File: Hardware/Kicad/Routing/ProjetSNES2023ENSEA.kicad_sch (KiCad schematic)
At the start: 43 parts, among them J1 Conn_01x07_Socket, Q1 2N7002, Q2 2N7002, Q3 2N7002, SW1 SW_Push, U1 NRF24L01, U2 AMS1117-3.3, U3 STM32L412KBTx, Y1 16 MHz

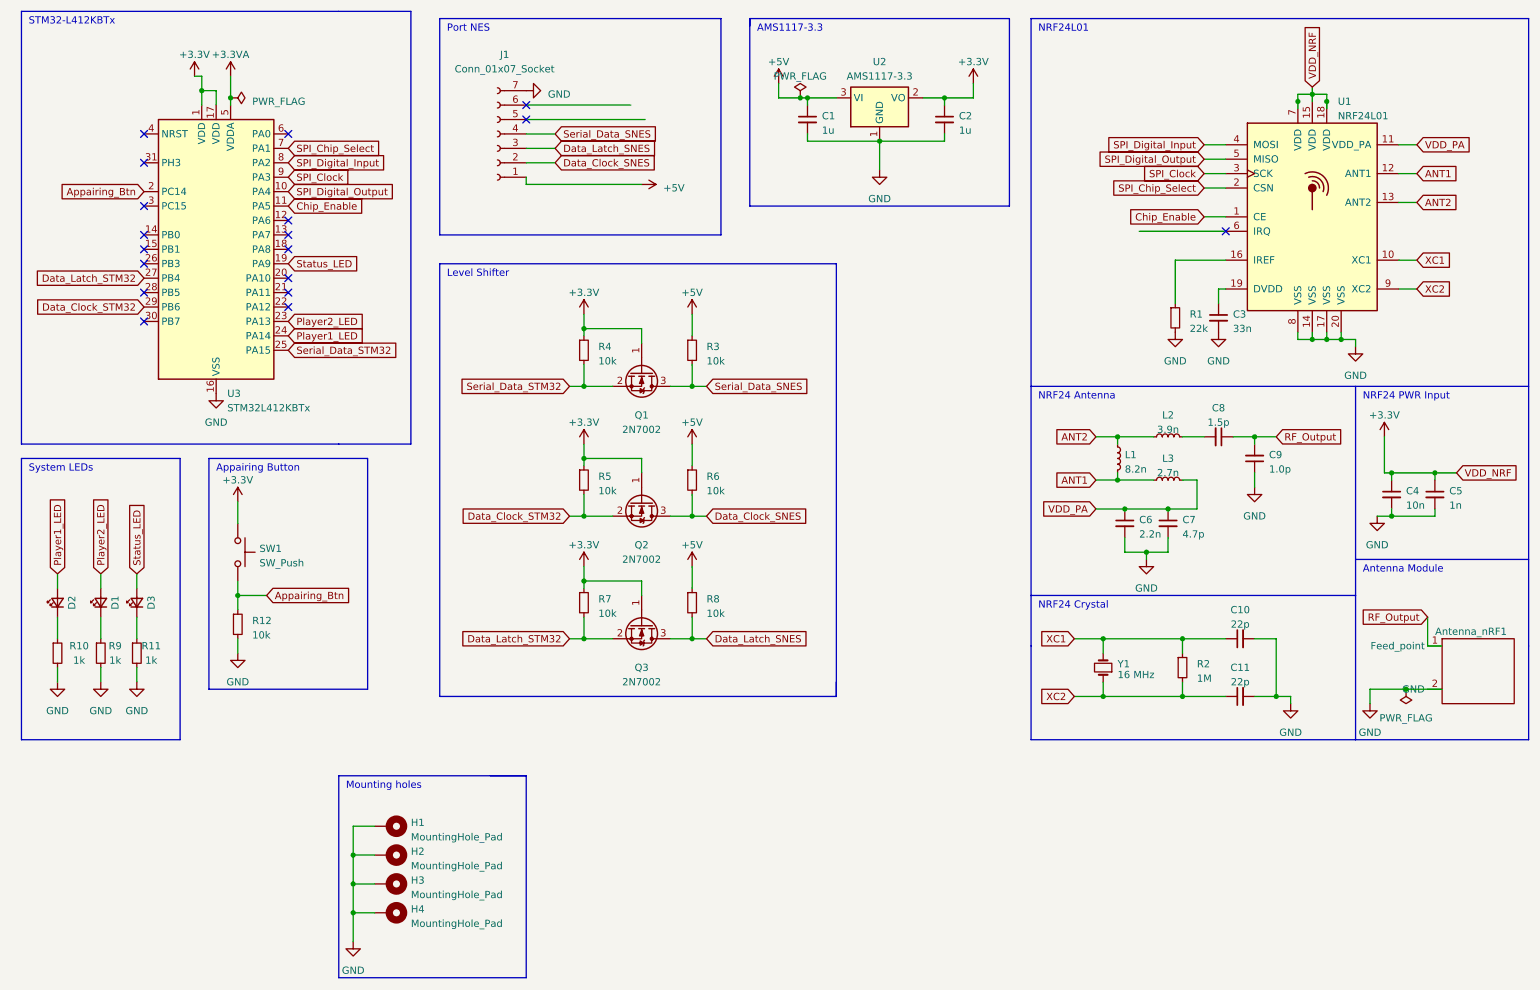
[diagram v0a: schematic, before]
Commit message: Updated Schematic & PCB
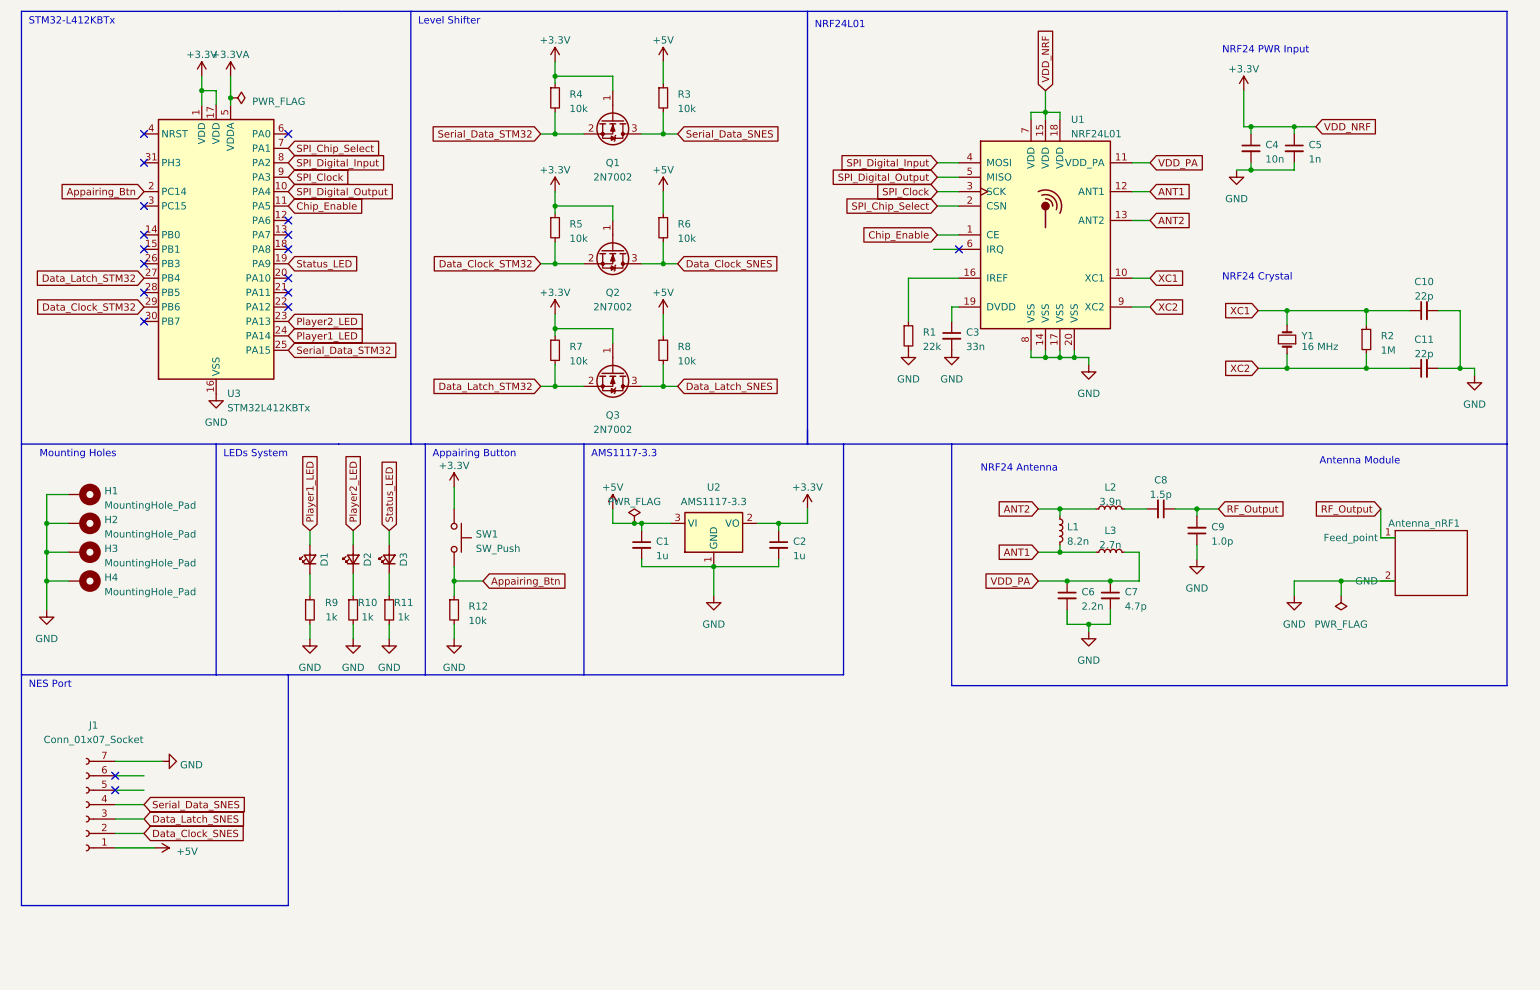
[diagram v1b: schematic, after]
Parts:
- renumbered D2 to D1, D1 to D2, R9 to R10, R10 to R9
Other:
- note added: "LEDs System"
- note added: "Mounting Holes"
- note added: "NES Port"
- note removed: "Mounting holes"
- note removed: "Port NES"
- note removed: "System LEDs"
- moved on the sheet: D1, D2, D3, H1, H2, H3, H4, Q1, Q2, Q3, R10, R11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
